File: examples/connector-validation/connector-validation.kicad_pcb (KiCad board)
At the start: 2 copper layers, 355.6 x 213.4 mm, 6 parts

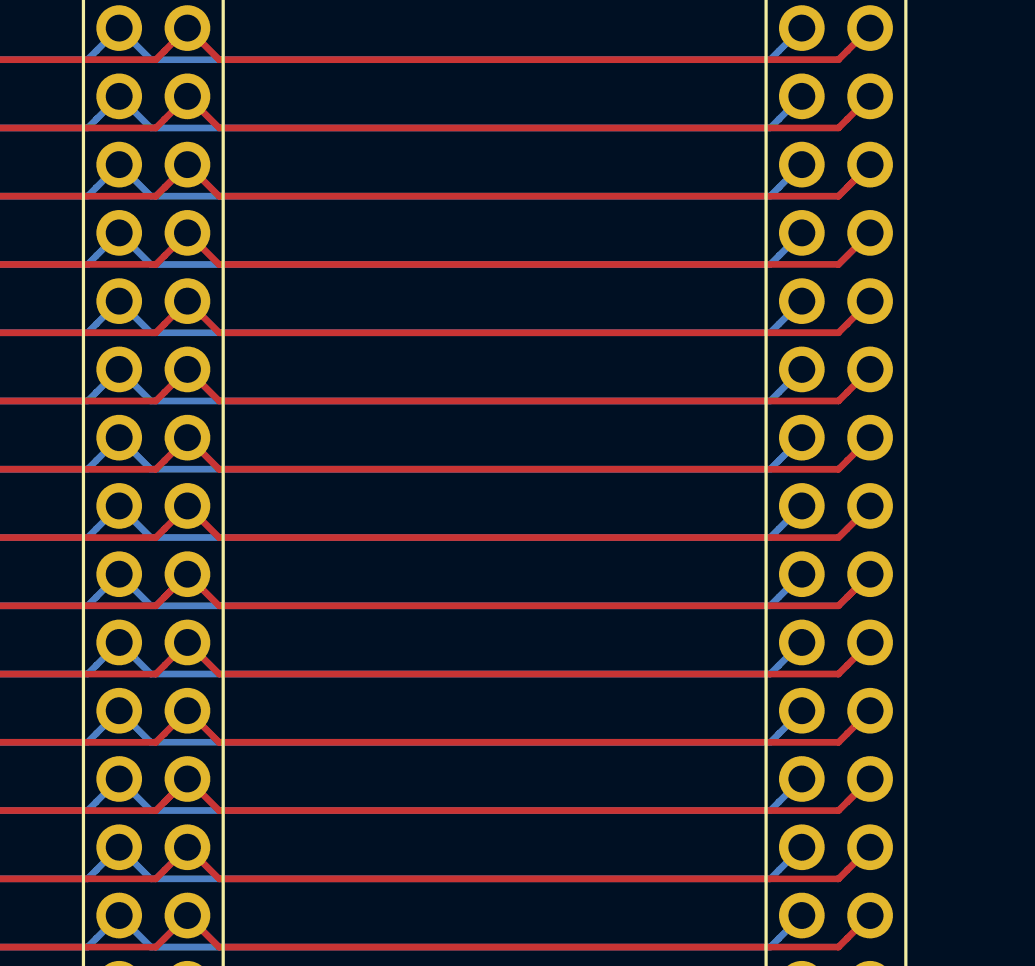
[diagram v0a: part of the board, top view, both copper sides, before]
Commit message: Linting fixes.
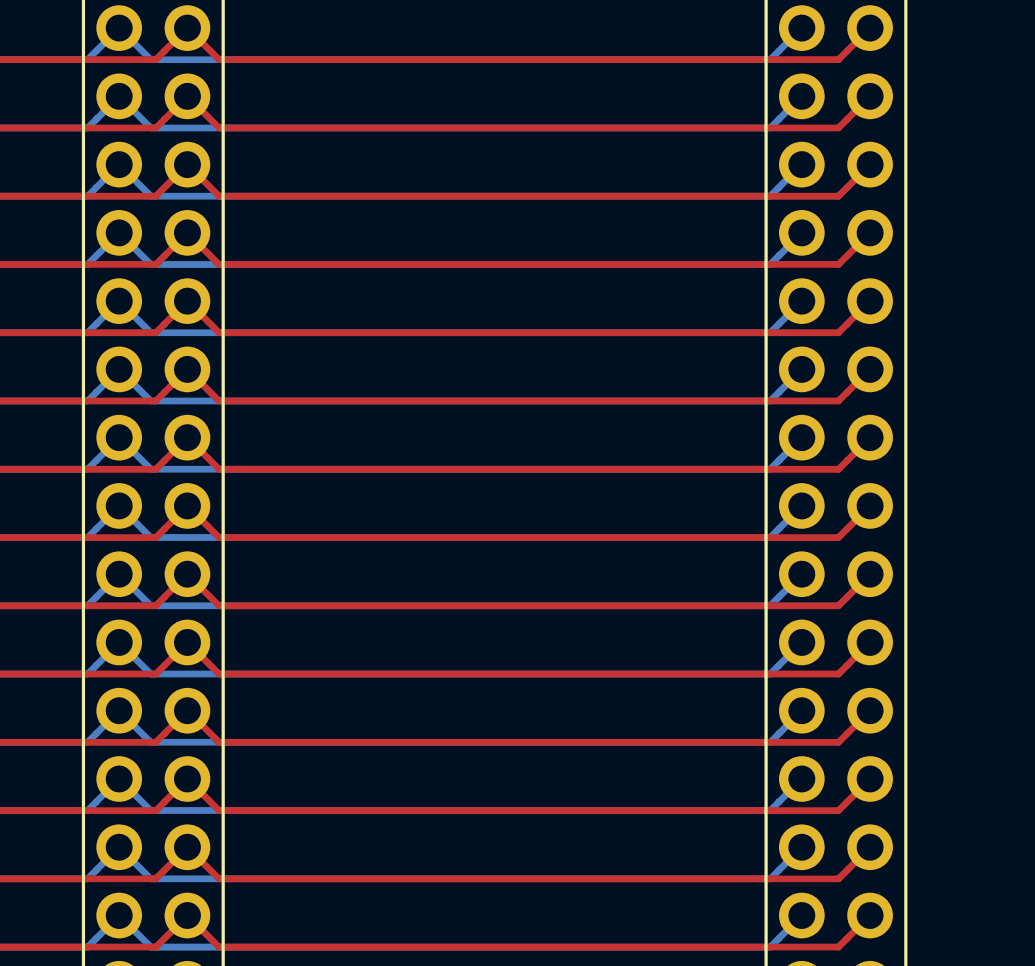
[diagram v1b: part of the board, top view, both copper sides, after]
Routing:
- net /backplane/BA09: track 55.2 -> 52.7 mm
- net /backplane/VCC: track 107.9 -> 105.5 mm
- net /backplane/BA15: track 55.2 -> 52.7 mm
